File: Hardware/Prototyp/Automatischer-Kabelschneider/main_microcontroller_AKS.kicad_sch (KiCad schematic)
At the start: 14 parts, among them J5 Conn_02x05_Odd_Even, SW1 SW_Push, SW2 SW_Push, U4 ESP32-S3-WROOM-2, U5 TMC2209_SILENTSTEPSTICK, U6 TMC2209_SILENTSTEPSTICK

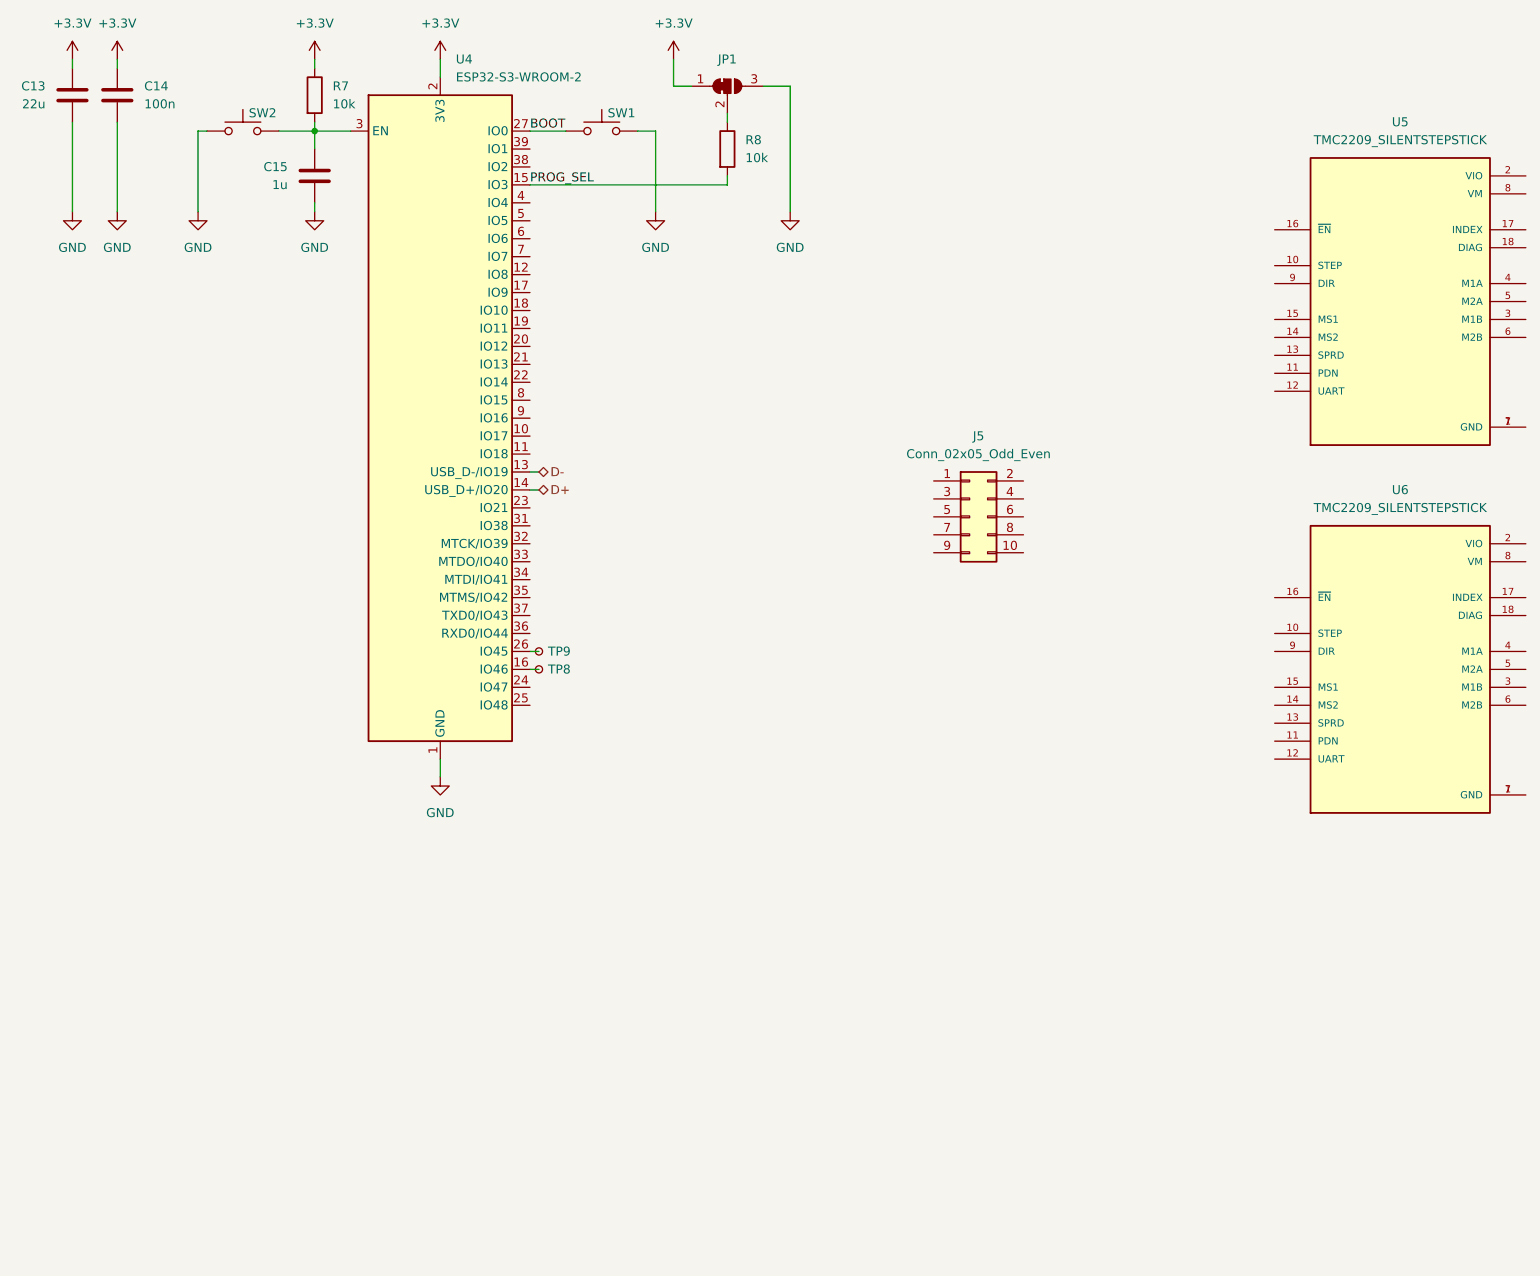
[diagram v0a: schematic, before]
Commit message: 20240501
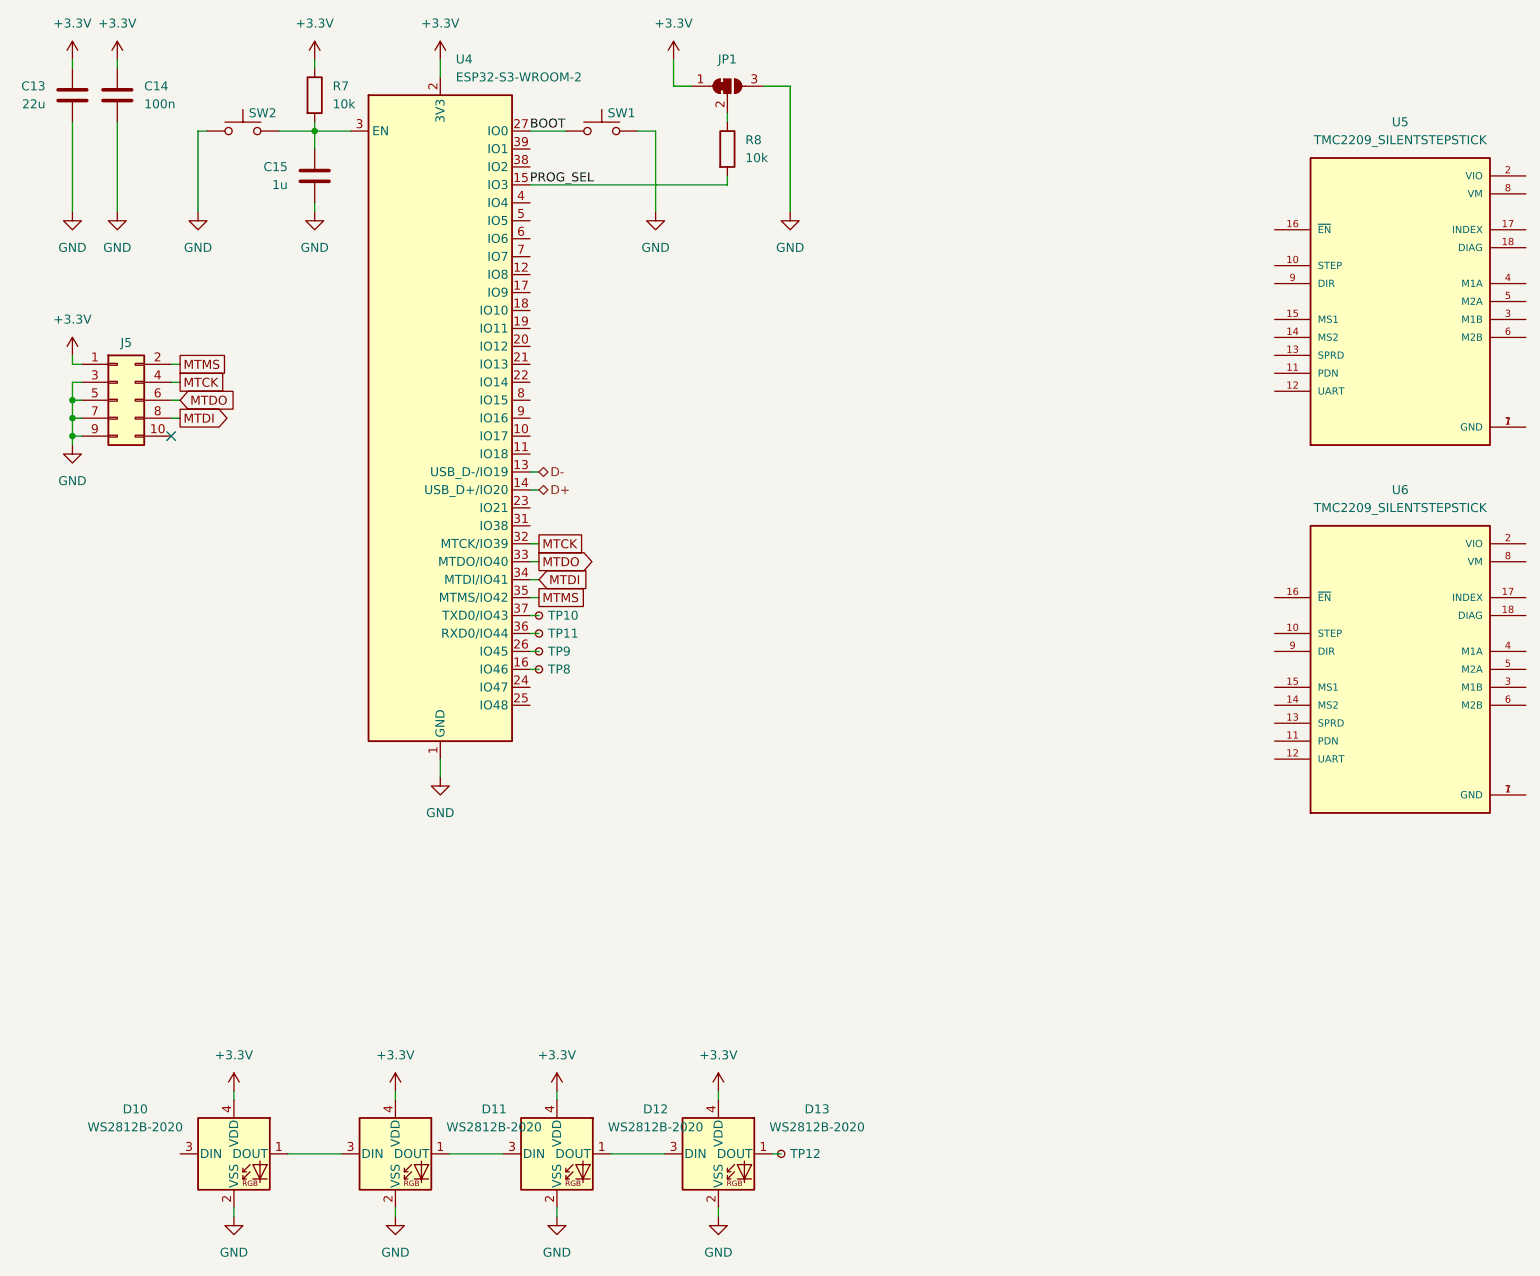
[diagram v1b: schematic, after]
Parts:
- added D10, D11, D12, D13: WS2812B-2020, LED_SMD:LED_WS2812B-2020_PLCC4_2.0x2.0mm, symbol LED:WS2812B-2020
- added TP10, TP11, TP12: TestPoint_Small, TestPoint:TestPoint_Pad_D1.0mm, symbol Connector:TestPoint_Small
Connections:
- net +3.3V: now also J5.1 (Pin_1), D10.4 (VDD), D11.4 (VDD), D12.4 (VDD), D13.4 (VDD)
- net GND: now also J5.3 (Pin_3), J5.5 (Pin_5), J5.7 (Pin_7), J5.9 (Pin_9), D10.2 (VSS), D11.2 (VSS), D12.2 (VSS), D13.2 (VSS)
- net MTMS: now reaches J5.2 (Pin_2)
- net MTMS: now also U4.35 (MTMS/IO42)
- net MTCK: now reaches J5.4 (Pin_4)
- net MTCK: now also U4.32 (MTCK/IO39)
- net MTDO: now reaches J5.6 (Pin_6)
- net MTDO: now also U4.33 (MTDO/IO40)
- net MTDI: now reaches J5.8 (Pin_8)
- net MTDI: now also U4.34 (MTDI/IO41)
- net at U4.36 (RXD0/IO44): now also TP11.1
- net at U4.37 (TXD0/IO43): now also TP10.1
- new net: D12.1 (DOUT), D13.3 (DIN)
- new net: D11.1 (DOUT), D12.3 (DIN)
- new net: D13.1 (DOUT), TP12.1
- new net: D10.1 (DOUT), D11.3 (DIN)
- no-connect marks 0 -> 1
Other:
- moved on the sheet: J5
